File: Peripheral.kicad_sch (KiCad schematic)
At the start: 5 parts, among them U2 AT24CS02-XHM, U3 ICM-20602, U6 ICM-4268-P

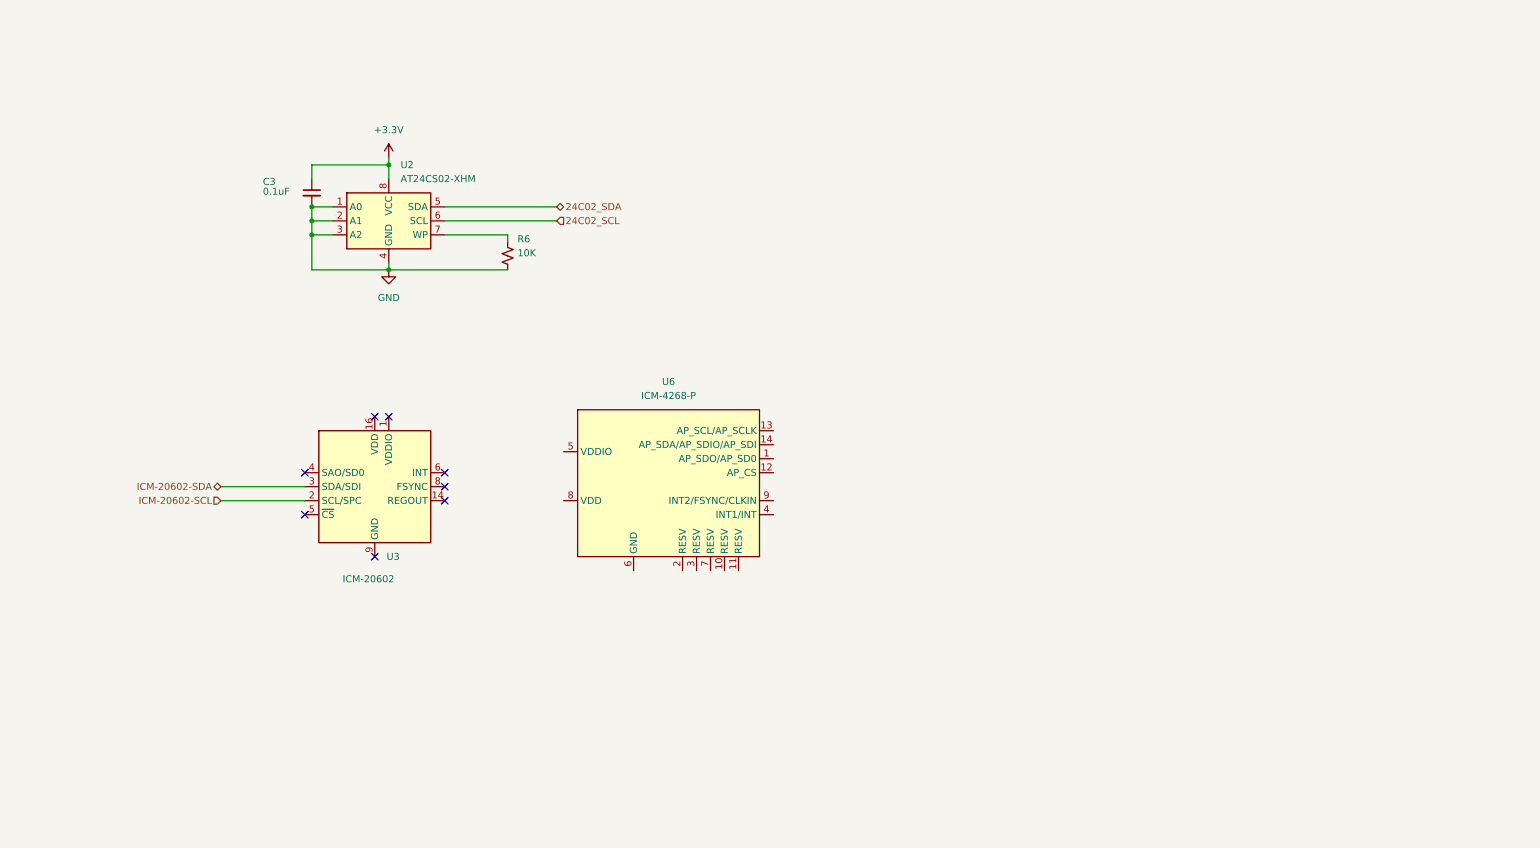
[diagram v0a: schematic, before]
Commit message: 优化IMU电路
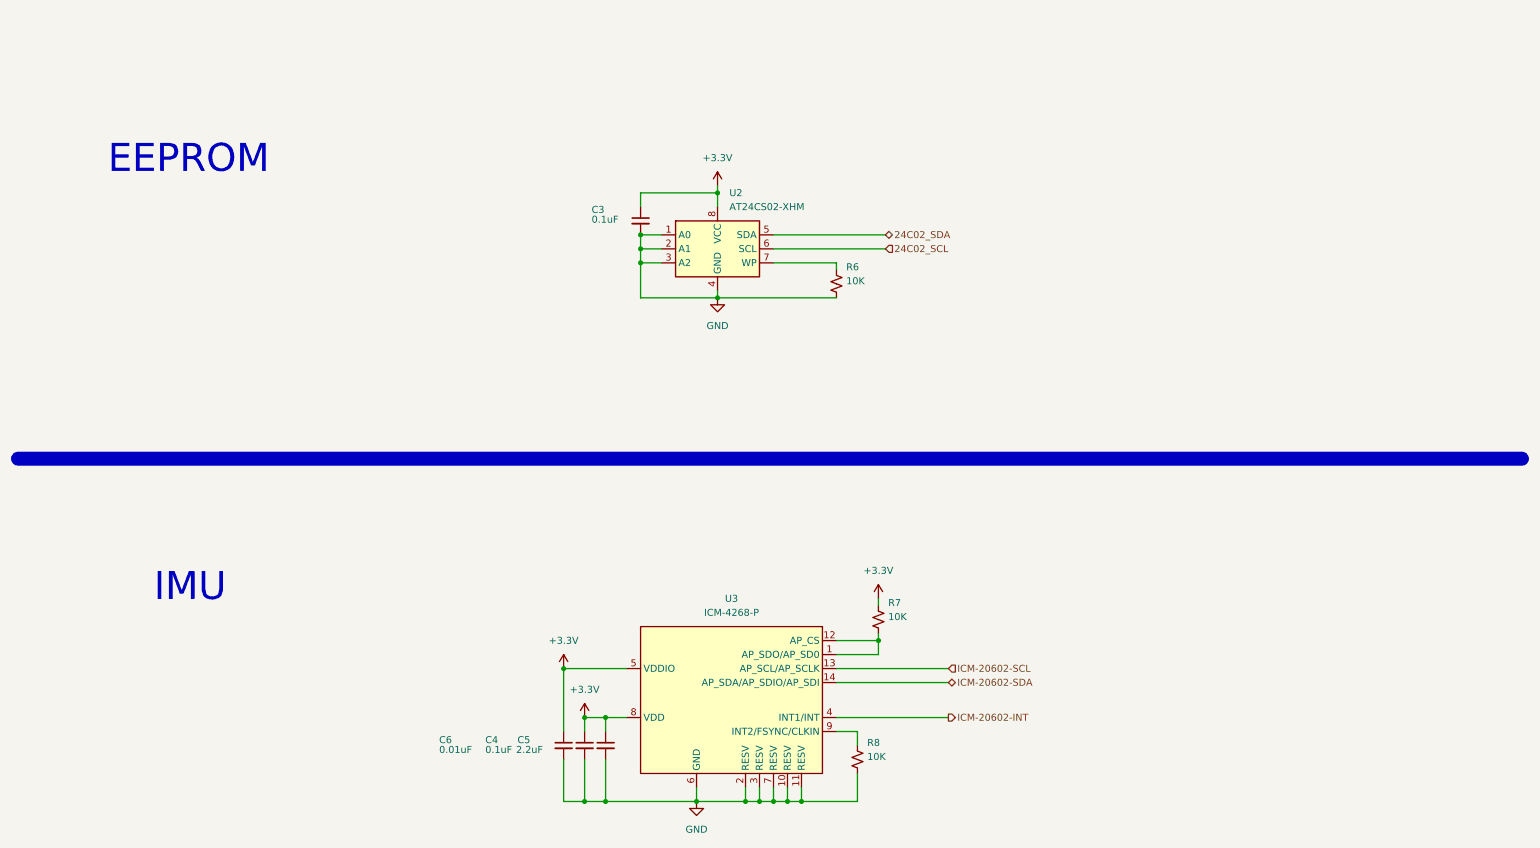
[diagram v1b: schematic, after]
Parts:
- removed U3: ICM-20602, Package_LGA:LGA-16_3x3mm_P0.5mm_LayoutBorder3x5y, symbol Sensor_Motion:ICM-20602
- removed U6: ICM-4268-P, Package_LGA:Bosch_LGA-14_3x2.5mm_P0.5mm, symbol User_Driver:ICM-42688-P
- added C4: 0.1uF, symbol Device:C_Small
- added C5: 2.2uF, symbol Device:C_Small
- added C6: 0.01uF, symbol Device:C_Small
- added R7, R8: 10K, symbol Device:R_Small_US
- added U3: ICM-4268-P, Package_LGA:Bosch_LGA-14_3x2.5mm_P0.5mm, symbol User_Driver:ICM-42688-P
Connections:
- net +3.3V: now also C4.1, C5.1, C6.1, R7.1, U3.5 (VDDIO), U3.8 (VDD)
- net GND: now also C4.2, C5.2, C6.2, R8.2, U3.10 (RESV), U3.11 (RESV), U3.2 (RESV), U3.3 (RESV), U3.6 (GND), U3.7 (RESV)
- net ICM-20602-SCL: now also U3.13 (AP_SCL/AP_SCLK)
- net ICM-20602-SDA: now also U3.14 (AP_SDA/AP_SDIO/AP_SDI)
- new net: R8.1, U3.9 (INT2/FSYNC/CLKIN)
- new net: R7.2, U3.1 (AP_SDO/AP_SD0), U3.12 (AP_CS)
- new net ICM-20602-INT: U3.4 (INT1/INT)
- no-connect marks 8 -> 0
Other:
- note added: "EEPROM"
- note added: "IMU"
- moved on the sheet: C3, R6, U2

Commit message: 优化接口
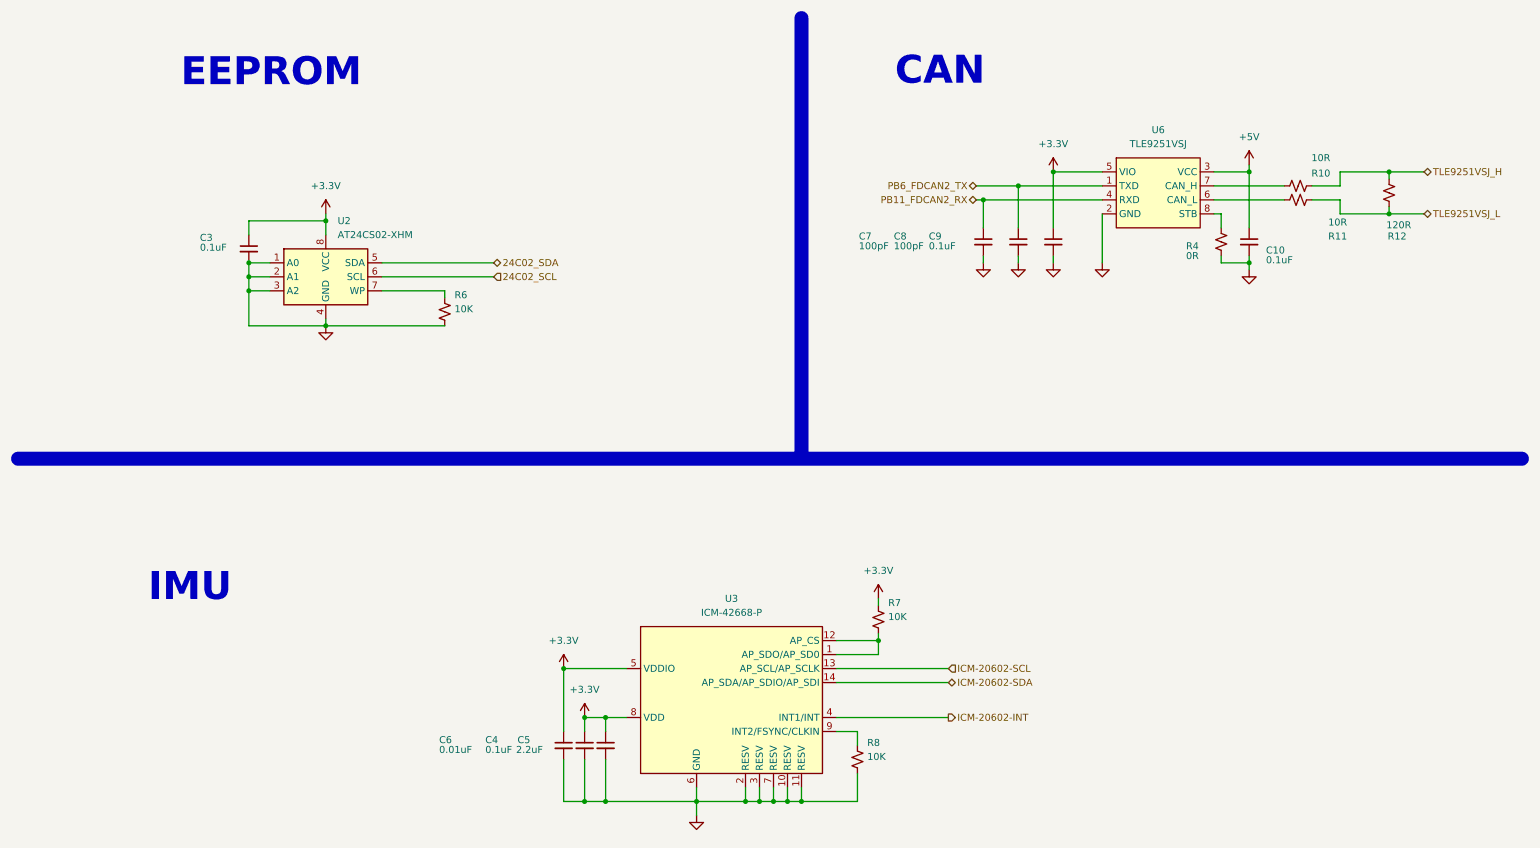
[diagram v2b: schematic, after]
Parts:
- added C10, C9: 0.1uF, Capacitor_SMD:C_0603_1608Metric_Pad1.08x0.95mm_HandSolder, symbol Device:C_Small
- added C7, C8: 100pF, Capacitor_SMD:C_0603_1608Metric_Pad1.08x0.95mm_HandSolder, symbol Device:C_Small
- added R10, R11: 10R, Resistor_SMD:R_0603_1608Metric_Pad0.98x0.95mm_HandSolder, symbol Device:R_Small_US
- added R12: 120R, Resistor_SMD:R_0603_1608Metric_Pad0.98x0.95mm_HandSolder, symbol Device:R_Small_US
- added R4: 0R, Resistor_SMD:R_0603_1608Metric_Pad0.98x0.95mm_HandSolder, symbol Device:R_Small_US
- added U6: TLE9251VSJ, Package_SO:Infineon_PG-DSO-8-24_4x5mm, symbol User_Driver:TLE9251VSJ
- C3, C4, C5, C6: footprint (none) -> Capacitor_SMD:C_0603_1608Metric_Pad1.08x0.95mm_HandSolder
- R6, R7, R8: footprint (none) -> Resistor_SMD:R_0603_1608Metric_Pad0.98x0.95mm_HandSolder
- U3: value ICM-4268-P -> ICM-42668-P
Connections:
- net +3.3V: now also C9.1, U6.5 (VIO)
- net GND: now also C10.2, C7.2, C8.2, C9.2, R4.1, U6.2 (GND)
- new net: R11.1, U6.6 (CAN_L)
- new net: R10.1, U6.7 (CAN_H)
- new net: R4.2, U6.8 (STB)
- new net +5V: C10.1, U6.3 (VCC)
- new net PB11_FDCAN2_RX: C7.1, U6.4 (RXD)
- new net PB6_FDCAN2_TX: C8.1, U6.1 (TXD)
- new net TLE9251VSJ_H: R10.2, R12.1
- new net TLE9251VSJ_L: R11.2, R12.2
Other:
- note added: "CAN"
- moved on the sheet: C3, R6, U2
